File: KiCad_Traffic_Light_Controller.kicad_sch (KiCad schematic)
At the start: 0 parts

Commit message: create schematic
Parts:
- added C1: 10u, symbol Device:C_Polarized_Small
- added C2, C3, C5: 0.22u, symbol Device:C_Small
- added C4: 100u, symbol Device:C_Polarized_Small
- added D1: NSC_GRN, symbol Device:LED
- added D10: EWP_RED, symbol Device:LED
- added D11, D12, D13: 1N4148W, Diode_SMD:D_SOD-123, symbol Diode:1N4148W
- added D2: NSC_YLW, symbol Device:LED
- added D3: NSC_RED, symbol Device:LED
- added D4: EWC_GRN, symbol Device:LED
- added D5: EWC_YLW, symbol Device:LED
- added D6: EWC_RED, symbol Device:LED
- added D7: NSP_GRN, symbol Device:LED
- added D8: NSP_RED, symbol Device:LED
- added D9: EWP_GRN, symbol Device:LED
- added H1, H2, H3, H4: MountingHole, symbol Mechanical:MountingHole
- added J1, J2: Conn_02x08_Odd_Even, symbol Connector_Generic:Conn_02x08_Odd_Even
- added J3: Conn_02x05_Odd_Even, symbol Connector_Generic:Conn_02x05_Odd_Even
- added J4: +5V, symbol Connector:Screw_Terminal_01x02
- added R1, R10, R11, R12, R13, R14, R15, R16, R17, R18, R19, R2, R20, R21, R22, R23, R24, R25, R26, R3, R4, R5, R6, R7, R8, R9: 130R, symbol Device:R_Small
- added R27, R28, R29, R30, R31, R32: 47K, symbol Device:R_Small
- added SW1: RST, symbol Switch:SW_Push
- added SW2: OVR, symbol Switch:SW_SPDT
- added SW3: EN, symbol Switch:SW_SPDT
- added U1, U2: SM420561N, Display_7Segment:7SegmentLED_LTS6760_LTS6780, symbol Display_Character:SM420561N
- added U3: LM1117DT-3.3, Package_TO_SOT_SMD:TO-252-3_TabPin2, symbol Regulator_Linear:LM1117DT-3.3
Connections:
- new net: D12.2 (A), R27.2, R29.2, SW1.2
- new net: D11.2 (A), R28.1, R30.2, SW2.2 (B)
- new net: D4.1 (K), R20.2
- new net: D13.2 (A), R31.1, R32.1, SW3.2 (B)
- new net: D7.1 (K), R23.2
- new net: D3.1 (K), R19.2
- new net: R2.2, U1.6 (B)
- new net: R6.2, U1.9 (F)
- new net: R5.2, U1.1 (E)
- new net: R11.2, U2.4 (C)
- new net: R13.2, U2.1 (E)
- new net: R15.2, U2.10 (G)
- new net: R12.2, U2.2 (D)
- new net: R16.2, U2.5 (DP)
- new net: R10.2, U2.6 (B)
- new net: R9.2, U2.7 (A)
- new net: R14.2, U2.9 (F)
- new net: D6.1 (K), R22.2
- new net: C5.1, D13.1 (K), R31.2
- new net: D1.1 (K), R17.2
- new net: R4.2, U1.2 (D)
- new net: D2.1 (K), R18.2
- new net: D5.1 (K), R21.2
- new net: D9.1 (K), R25.2
- new net: R8.2, U1.5 (DP)
- new net: R1.2, U1.7 (A)
- new net: D10.1 (K), R26.2
- new net: D8.1 (K), R24.2
- new net: R7.2, U1.10 (G)
- new net: R3.2, U1.4 (C)
- new net +3.3V: C4.1, J1.1 (Pin_1), J2.1 (Pin_1), R27.1, R30.1, R32.2, U3.2 (VO)
- new net +5V: C1.1, J3.7 (Pin_7), J3.9 (Pin_9), J4.2 (Pin_2), U3.3 (VI)
- new net EN: J3.3 (Pin_3)
- new net EWC_GRN: D4.2 (A), J2.3 (Pin_3)
- new net EWC_RED: D6.2 (A), J2.7 (Pin_7)
- new net EWC_YLW: D5.2 (A), J2.5 (Pin_5)
- new net EWP_GRN: D9.2 (A), J2.6 (Pin_6)
- new net EWP_RED: D10.2 (A), J2.8 (Pin_8)
- new net EW_HEX_A: J2.9 (Pin_9), R9.1
- new net EW_HEX_B: J2.11 (Pin_11), R10.1
- new net EW_HEX_C: J2.13 (Pin_13), R11.1
- new net EW_HEX_D: J2.15 (Pin_15), R12.1
- new net EW_HEX_DP: J2.16 (Pin_16), R16.1
- new net EW_HEX_E: J2.10 (Pin_10), R13.1
- new net EW_HEX_F: J2.12 (Pin_12), R14.1
- new net EW_HEX_G: J2.14 (Pin_14), R15.1
- new net GND: C1.2, C2.2, C3.2, C4.2, C5.2, J1.2 (Pin_2), J1.4 (Pin_4), J2.2 (Pin_2), J2.4 (Pin_4), J3.10 (Pin_10), J3.2 (Pin_2), J3.4 (Pin_4), J3.6 (Pin_6), J3.8 (Pin_8), J4.1 (Pin_1), R17.1, R18.1, R19.1, R20.1, R21.1, R22.1, R23.1, R24.1, R25.1, R26.1, SW1.1, SW2.3 (C), SW3.3 (C), U1.3 (CC), U1.8 (CC), U2.3 (CC), U2.8 (CC), U3.1 (GND)
- new net NSC_GRN: D1.2 (A), J1.3 (Pin_3)
- new net NSC_RED: D3.2 (A), J1.7 (Pin_7)
- new net NSC_YLW: D2.2 (A), J1.5 (Pin_5)
- new net NSP_GRN: D7.2 (A), J1.6 (Pin_6)
- new net NSP_RED: D8.2 (A), J1.8 (Pin_8)
- new net NS_HEX_A: J1.9 (Pin_9), R1.1
- new net NS_HEX_B: J1.11 (Pin_11), R2.1
- new net NS_HEX_C: J1.13 (Pin_13), R3.1
- new net NS_HEX_D: J1.15 (Pin_15), R4.1
- new net NS_HEX_DP: J1.16 (Pin_16), R8.1
- new net NS_HEX_E: J1.10 (Pin_10), R5.1
- new net NS_HEX_F: J1.12 (Pin_12), R6.1
- new net NS_HEX_G: J1.14 (Pin_14), R7.1
- new net OVR: C2.1, D11.1 (K), J3.5 (Pin_5), R28.2
- new net RST: C3.1, D12.1 (K), J3.1 (Pin_1), R29.1
- no-connect marks 0 -> 2
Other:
- note added: "+3.3V VOLTAGE REGULATOR"
- note added: "CAR TRAFFIC LIGHTS"
- note added: "CONNECTORS"
- note added: "CONTROL LOGIC"
- note added: "EAST-WEST TRAFFIC LIGHT"
- note added: "EMERGENCY OVERRIDE"
- note added: "ENABLE"
- note added: "MOUNTING HOLES"
- note added: "NORTH-SOUTH TRAFFIC LIGHT"
- note added: "PEDESTRIAN TRAFFIC LIGHTS"
- note added: "RESET"
- note added: "TIMER"

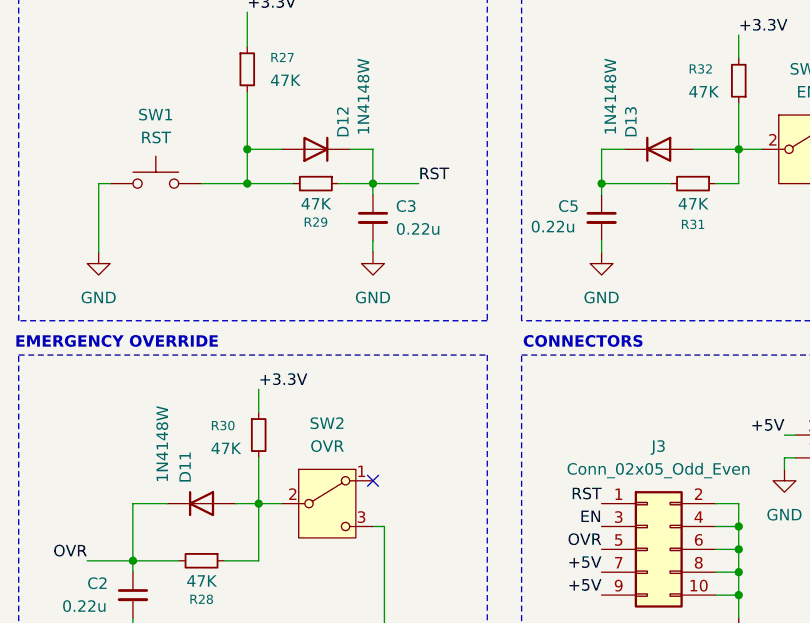
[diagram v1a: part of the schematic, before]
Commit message: create pcb design
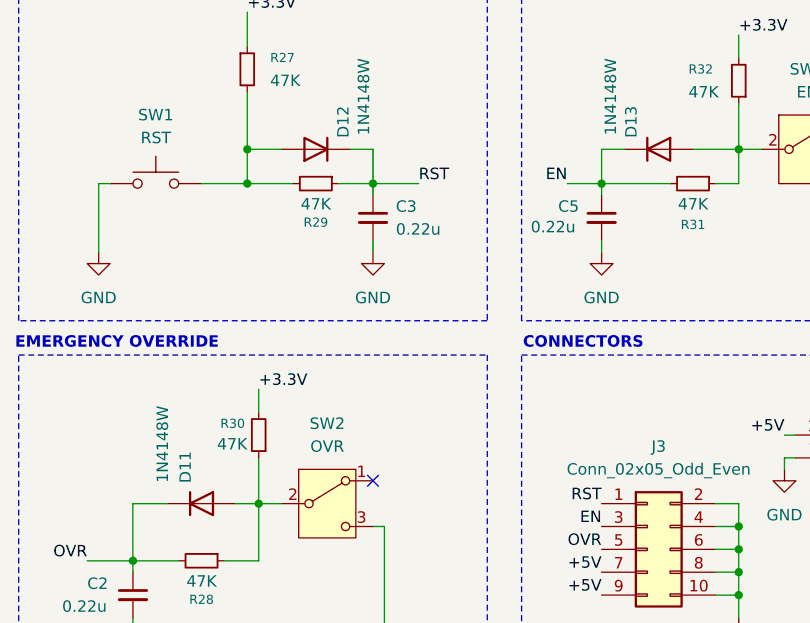
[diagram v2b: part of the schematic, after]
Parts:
- C1: footprint (none) -> Capacitor_SMD:CP_Elec_4x5.3
- C2, C3, C5: footprint (none) -> Capacitor_SMD:C_1206_3216Metric_Pad1.33x1.80mm_HandSolder
- C4: footprint (none) -> Capacitor_SMD:CP_Elec_6.3x5.8
- D1, D10, D2, D3, D4, D5, D6, D7, D8, D9: footprint (none) -> LED_THT:LED_D5.0mm
- H1, H2, H3, H4: footprint (none) -> MountingHole:MountingHole_2.2mm_M2
- J1, J2: footprint (none) -> Connector_PinHeader_2.54mm:PinHeader_2x08_P2.54mm_Vertical
- J3: footprint (none) -> Connector_PinHeader_2.54mm:PinHeader_2x05_P2.54mm_Vertical
- J4: footprint (none) -> my_footprints:Terminal_Block_5mm
- R1, R10, R11, R12, R13, R14, R15, R16, R17, R18, R19, R2, R20, R21, R22, R23, R24, R25, R26, R27, R28, R29, R3, R30, R31, R32, R4, R5, R6, R7, R8, R9: footprint (none) -> Resistor_SMD:R_1206_3216Metric_Pad1.30x1.75mm_HandSolder
- SW1: footprint (none) -> my_footprints:tact_switch_5mm
- SW2, SW3: footprint (none) -> my_footprints:slide_switch_2.54mm
- U3: footprint Package_TO_SOT_SMD:TO-252-3_TabPin2 -> Package_TO_SOT_SMD:SOT-223
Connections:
- net +3.3V: now also R30.2; no longer R30.1
- net EN: now also C5.1, D13.1 (K), R31.2
- net at D11.2 (A), R28.1, SW2.2 (B): now also R30.1; no longer R30.2
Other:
- moved on the sheet: R30
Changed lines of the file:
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@@
 	(wire
 		(pts
+			(xy 243.84 62.23) (xy 247.65 62.23)
+		)
+		(stroke
+			(width 0)
+			(type default)
+		)
+	)
+	(wire
+		(pts
 			(xy 53.34 67.31) (xy 55.88 67.31)
 		)
@@
 		)
 	)
+	(label "EN"
+		(at 243.84 62.23 180)
+		(effects
+			(font
+				(size 1.27 1.27)
+			)
+			(justify right bottom)
+		)
+	)
 	(label "EW_HEX_F"
 		(at 162.56 115.57 0)
@@
 			)
 		)
-		(property "Footprint" ""
+		(property "Footprint" "Resistor_SMD:R_1206_3216Metric_Pad1.30x1.75mm_HandSolder"
 			(at 208.28 49.53 0)
 			(effects
@@
 			)
 		)
-		(property "Footprint" ""
+		(property "Footprint" "Resistor_SMD:R_1206_3216Metric_Pad1.30x1.75mm_HandSolder"
 			(at 72.39 99.06 0)
 			(effects
@@
 			)
 		)
-		(property "Footprint" ""
+		(property "Footprint" "my_footprints:slide_switch_2.54mm"
 			(at 217.17 97.79 0)
 			(effects
@@
 			)
 		)
-		(property "Footprint" ""
+		(property "Footprint" "Resistor_SMD:R_1206_3216Metric_Pad1.30x1.75mm_HandSolder"
 			(at 262.89 50.8 0)
 			(effects
@@
 			)
 		)
-		(property "Footprint" ""
+		(property "Footprint" "Resistor_SMD:R_1206_3216Metric_Pad1.30x1.75mm_HandSolder"
 			(at 110.49 52.07 0)
 			(effects
@@
 			)
 		)
-		(property "Footprint" ""
+		(property "Footprint" "Resistor_SMD:R_1206_3216Metric_Pad1.30x1.75mm_HandSolder"
 			(at 72.39 68.58 0)
 			(effects
@@
 			)
 		)
-		(property "Footprint" ""
+		(property "Footprint" "Resistor_SMD:R_1206_3216Metric_Pad1.30x1.75mm_HandSolder"
 			(at 33.02 54.61 0)
 			(effects
@@
 			)
 		)
-		(property "Footprint" ""
+		(property "Footprint" "Connector_PinHeader_2.54mm:PinHeader_2x05_P2.54mm_Vertical"
 			(at 252.73 102.87 0)
 			(effects
@@
 			)
 		)
-		(property "Footprint" ""
+		(property "Footprint" "Resistor_SMD:R_1206_3216Metric_Pad1.30x1.75mm_HandSolder"
 			(at 33.02 64.77 0)
 			(effects
@@
 			)
 		)
-		(property "Footprint" ""
+		(property "Footprint" "LED_THT:LED_D5.0mm"
 			(at 83.82 68.58 0)
 			(effects
@@
 			)
 		)
-		(property "Footprint" ""
+		(property "Footprint" "MountingHole:MountingHole_2.2mm_M2"
 			(at 246.38 140.97 0)
 			(effects
@@
 			)
 		)
-		(property "Footprint" ""
+		(property "Footprint" "Resistor_SMD:R_1206_3216Metric_Pad1.30x1.75mm_HandSolder"
 			(at 33.02 62.23 0)
 			(effects
@@
 			)
 		)
-		(property "Footprint" ""
+		(property "Footprint" "Resistor_SMD:R_1206_3216Metric_Pad1.30x1.75mm_HandSolder"
 			(at 33.02 107.95 0)
 			(effects
@@
 			)
 		)
-		(property "Footprint" ""
+		(property "Footprint" "Capacitor_SMD:CP_Elec_6.3x5.8"
 			(at 222.25 138.43 0)
 			(effects
@@
 			)
 		)
-		(property "Footprint" ""
+		(property "Footprint" "Capacitor_SMD:C_1206_3216Metric_Pad1.33x1.80mm_HandSolder"
 			(at 222.25 66.04 0)
 			(effects
@@
 			)
 		)
-		(property "Footprint" ""
+		(property "Footprint" "LED_THT:LED_D5.0mm"
 			(at 83.82 119.38 0)
 			(effects
@@
 			)
 		)
-		(property "Footprint" ""
+		(property "Footprint" "Resistor_SMD:R_1206_3216Metric_Pad1.30x1.75mm_HandSolder"
 			(at 257.81 62.23 0)
 			(effects
@@
 			)
 		)
-		(property "Footprint" ""
+		(property "Footprint" "Resistor_SMD:R_1206_3216Metric_Pad1.30x1.75mm_HandSolder"
 			(at 72.39 48.26 0)
 			(effects
@@
 			)
 		)
-		(property "Footprint" ""
+		(property "Footprint" "Resistor_SMD:R_1206_3216Metric_Pad1.30x1.75mm_HandSolder"
 			(at 33.02 59.69 0)
 			(effects
@@
 			)
 		)
-		(property "Footprint" ""
+		(property "Footprint" "Resistor_SMD:R_1206_3216Metric_Pad1.30x1.75mm_HandSolder"
 			(at 33.02 115.57 0)
 			(effects
@@
 			)
 		)
-		(property "Footprint" ""
+		(property "Footprint" "MountingHole:MountingHole_2.2mm_M2"
 			(at 246.38 147.32 0)
 			(effects
@@
 			)
 		)
-		(property "Footprint" ""
+		(property "Footprint" "LED_THT:LED_D5.0mm"
 			(at 121.92 52.07 0)
 			(effects
@@
 			)
 		)
-		(property "Footprint" ""
+		(property "Footprint" "Resistor_SMD:R_1206_3216Metric_Pad1.30x1.75mm_HandSolder"
 			(at 33.02 120.65 0)
 			(effects
@@
 			)
 		)
-		(property "Footprint" ""
+		(property "Footprint" "Resistor_SMD:R_1206_3216Metric_Pad1.30x1.75mm_HandSolder"
 			(at 215.9 62.23 0)
 			(effects
@@
 			)
 		)
-		(property "Footprint" ""
+		(property "Footprint" "Resistor_SMD:R_1206_3216Metric_Pad1.30x1.75mm_HandSolder"
 			(at 33.02 105.41 0)
 			(effects
@@
 			)
 		)
-		(property "Footprint" ""
+		(property "Footprint" "Resistor_SMD:R_1206_3216Metric_Pad1.30x1.75mm_HandSolder"
 			(at 72.39 58.42 0)
 			(effects
@@
 			)
 		)
-		(property "Footprint" ""
+		(property "Footprint" "Capacitor_SMD:C_1206_3216Metric_Pad1.33x1.80mm_HandSolder"
 			(at 247.65 66.04 0)
 			(effects
@@
 			)
 		)
-		(property "Footprint" ""
+		(property "Footprint" "LED_THT:LED_D5.0mm"
 			(at 83.82 109.22 0)
 			(effects
@@
 			)
 		)
-		(property "Footprint" ""
+		(property "Footprint" "Connector_PinHeader_2.54mm:PinHeader_2x08_P2.54mm_Vertical"
 			(at 154.94 59.69 0)
 			(effects
@@
 			)
 		)
-		(property "Footprint" ""
+		(property "Footprint" "LED_THT:LED_D5.0mm"
 			(at 121.92 102.87 0)
 			(effects
@@
 			)
 		)
-		(property "Footprint" ""
+		(property "Footprint" "Resistor_SMD:R_1206_3216Metric_Pad1.30x1.75mm_HandSolder"
 			(at 72.39 109.22 0)
 			(effects
@@
 			)
 		)
-		(property "Footprint" ""
+		(property "Footprint" "Resistor_SMD:R_1206_3216Metric_Pad1.30x1.75mm_HandSolder"
 			(at 110.49 102.87 0)
 			(effects
@@
 			)
 		)
-		(property "Footprint" ""
+		(property "Footprint" "Resistor_SMD:R_1206_3216Metric_Pad1.30x1.75mm_HandSolder"
 			(at 33.02 69.85 0)
 			(effects
@@
 			)
 		)
-		(property "Footprint" ""
+		(property "Footprint" "Capacitor_SMD:CP_Elec_4x5.3"
 			(at 193.04 138.43 0)
 			(effects
@@
 			)
 		)
-		(property "Footprint" ""
+		(property "Footprint" "Connector_PinHeader_2.54mm:PinHeader_2x08_P2.54mm_Vertical"
 			(at 154.94 110.49 0)
 			(effects
@@
 			)
 		)
-		(property "Footprint" ""
+		(property "Footprint" "LED_THT:LED_D5.0mm"
 			(at 83.82 48.26 0)
 			(effects
@@
 			)
 		)
-		(property "Footprint" ""
+		(property "Footprint" "my_footprints:Terminal_Block_5mm"
 			(at 274.32 92.71 0)
 			(effects
@@
 			)
 		)
-		(property "Footprint" ""
+		(property "Footprint" "Resistor_SMD:R_1206_3216Metric_Pad1.30x1.75mm_HandSolder"
 			(at 72.39 119.38 0)
 			(effects
@@
 			)
 		)
-		(property "Footprint" "Package_TO_SOT_SMD:TO-252-3_TabPin2"
+		(property "Footprint" "Package_TO_SOT_SMD:SOT-223"
 			(at 208.28 133.35 0)
 			(effects
@@
 			)
 		)
-		(property "Footprint" ""
+		(property "Footprint" "Resistor_SMD:R_1206_3216Metric_Pad1.30x1.75mm_HandSolder"
 			(at 33.02 118.11 0)
 			(effects
@@
 			)
 		)
-		(property "Footprint" ""
+		(property "Footprint" "Resistor_SMD:R_1206_3216Metric_Pad1.30x1.75mm_HandSolder"
 			(at 33.02 52.07 0)
 			(effects
@@
 			)
 		)
-		(property "Footprint" ""
+		(property "Footprint" "Resistor_SMD:R_1206_3216Metric_Pad1.30x1.75mm_HandSolder"
 			(at 33.02 110.49 0)
 			(effects
@@
 			)
 		)
-		(property "Footprint" ""
+		(property "Footprint" "Resistor_SMD:R_1206_3216Metric_Pad1.30x1.75mm_HandSolder"
 			(at 203.2 104.14 0)
 			(effects
@@
 			)
 		)
-		(property "Footprint" ""
+		(property "Footprint" "LED_THT:LED_D5.0mm"
 			(at 83.82 99.06 0)
 			(effects
@@
 			)
 		)
-		(property "Footprint" ""
+		(property "Footprint" "Resistor_SMD:R_1206_3216Metric_Pad1.30x1.75mm_HandSolder"
 			(at 110.49 113.03 0)
 			(effects
@@
 			)
 		)
-		(property "Footprint" ""
+		(property "Footprint" "MountingHole:MountingHole_2.2mm_M2"
 			(at 246.38 128.27 0)
 			(effects
@@
 			)
 		)
-		(property "Footprint" ""
+		(property "Footprint" "LED_THT:LED_D5.0mm"
 			(at 121.92 113.03 0)
 			(effects
@@
 	(symbol
 		(lib_id "Device:R_Small")
-		(at 209.55 90.17 0)
+		(at 209.55 90.17 180)
 		(unit 1)
 		(exclude_from_sim no)
@@
 		(dnp no)
 		(property "Reference" "R30"
-			(at 204.216 89.154 0)
+			(at 208.026 88.9 0)
 			(effects
 				(font
@@
 		)
 		(property "Value" "47K"
-			(at 204.216 91.694 0)
+			(at 208.28 91.186 0)
 			(effects
 				(font
@@
 			)
 		)
-		(property "Footprint" ""
+		(property "Footprint" "Resistor_SMD:R_1206_3216Metric_Pad1.30x1.75mm_HandSolder"
 			(at 209.55 90.17 0)
 			(effects
@@
 		)
 		(instances
-			(project ""
+			(project "KiCad_Traffic_Light_Controller"
 				(path "/72e88c87-4cdb-42c5-a385-70698eb55c38"
 					(reference "R30")
@@
 			)
 		)
-		(property "Footprint" ""
+		(property "Footprint" "Capacitor_SMD:C_1206_3216Metric_Pad1.33x1.80mm_HandSolder"
 			(at 195.58 107.95 0)
 			(effects
@@
 			)
 		)
-		(property "Footprint" ""
+		(property "Footprint" "my_footprints:slide_switch_2.54mm"
 			(at 270.51 58.42 0)
 			(effects
@@
 			)
 		)
-		(property "Footprint" ""
+		(property "Footprint" "my_footprints:tact_switch_5mm"
 			(at 198.12 57.15 0)
 			(effects
@@
 			)
 		)
-		(property "Footprint" ""
+		(property "Footprint" "LED_THT:LED_D5.0mm"
 			(at 121.92 62.23 0)
 			(effects
@@
 			)
 		)
-		(property "Footprint" ""
+		(property "Footprint" "Resistor_SMD:R_1206_3216Metric_Pad1.30x1.75mm_HandSolder"
 			(at 33.02 67.31 0)
 			(effects
@@
 			)
 		)
-		(property "Footprint" ""
+		(property "Footprint" "Resistor_SMD:R_1206_3216Metric_Pad1.30x1.75mm_HandSolder"
 			(at 33.02 113.03 0)
 			(effects
@@
 			)
 		)
-		(property "Footprint" ""
+		(property "Footprint" "LED_THT:LED_D5.0mm"
 			(at 83.82 58.42 0)
 			(effects
@@
 			)
 		)
-		(property "Footprint" ""
+		(property "Footprint" "Resistor_SMD:R_1206_3216Metric_Pad1.30x1.75mm_HandSolder"
 			(at 33.02 57.15 0)
 			(effects
@@
 			)
 		)
-		(property "Footprint" ""
+		(property "Footprint" "Resistor_SMD:R_1206_3216Metric_Pad1.30x1.75mm_HandSolder"
 			(at 33.02 102.87 0)
 			(effects
@@
 			)
 		)
-		(property "Footprint" ""
+		(property "Footprint" "MountingHole:MountingHole_2.2mm_M2"
 			(at 246.38 134.62 0)
 			(effects
@@
 			)
 		)
-		(property "Footprint" ""
+		(property "Footprint" "Resistor_SMD:R_1206_3216Metric_Pad1.30x1.75mm_HandSolder"
 			(at 110.49 62.23 0)
 			(effects
